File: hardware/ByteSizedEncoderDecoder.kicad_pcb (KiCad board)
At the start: 2 copper layers, 21.6 x 25.4 mm, 17 parts, among them J1 BM04B-SRSS-TB_LF__SN_, J10 1x4 female header pins 0.1", J11 ICSP pads, J2 BM04B-SRSS-TB_LF__SN_, J3 1x4 female header pins 0.1", J4 1x4 female header pins 0.1", J5 1x4 female header pins 0.1", J6 1x4 female header pins 0.1", J7 1x4 female header pins 0.1", J8 1x4 female header pins 0.1", J9 1x4 female header pins 0.1", U1 ATMEGA328PB

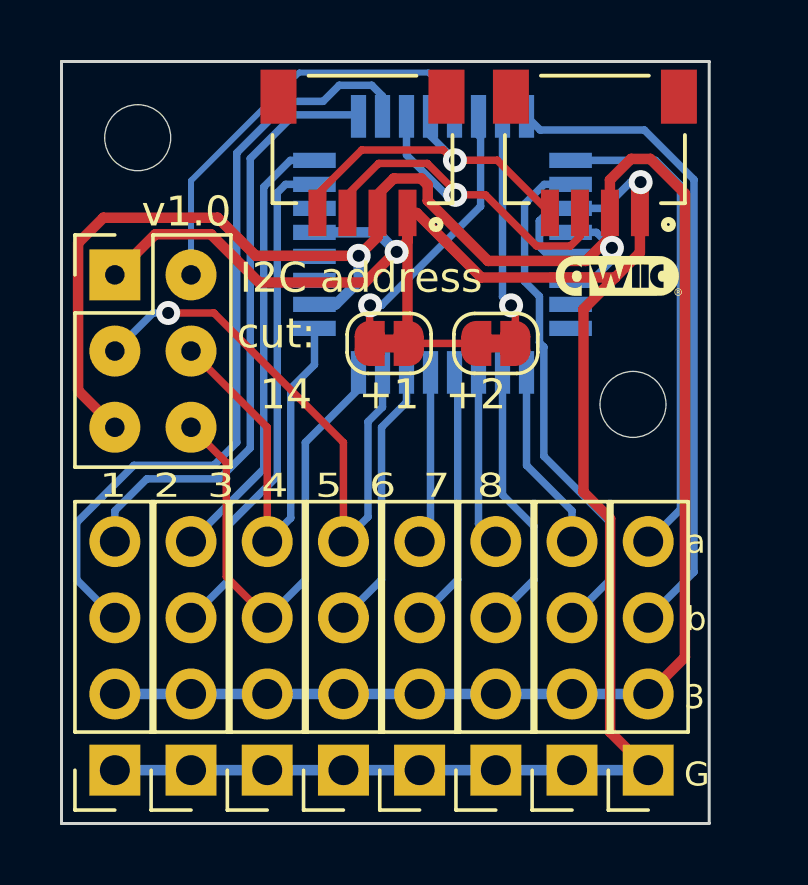
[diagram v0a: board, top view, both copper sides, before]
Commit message: v1.0
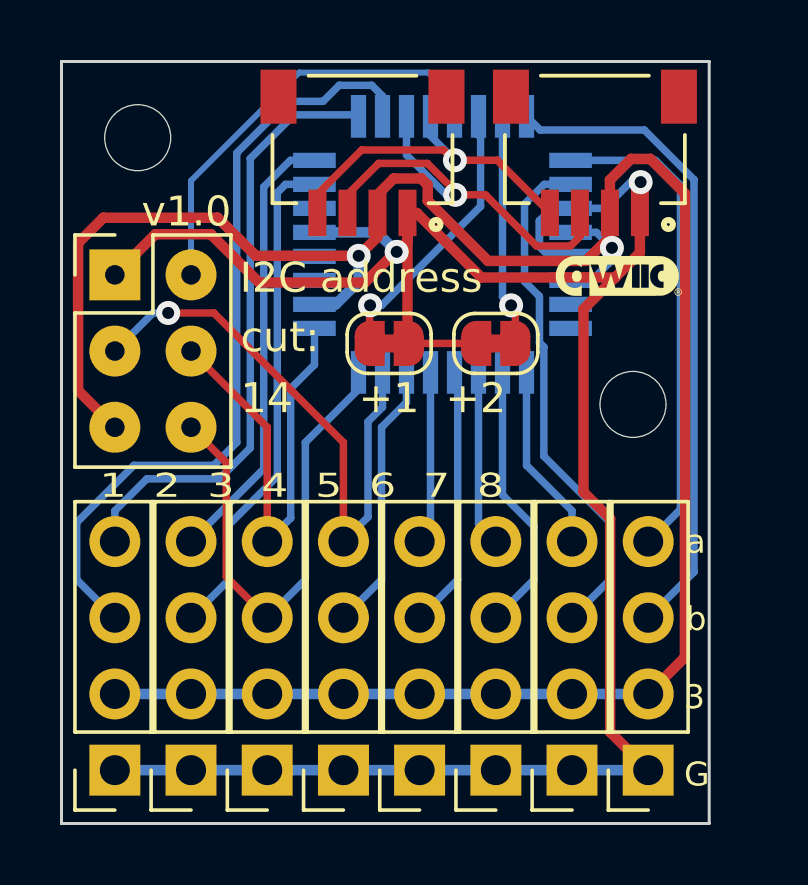
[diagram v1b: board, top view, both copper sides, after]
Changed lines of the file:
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@@
       (plotinvisibletext false)
       (sketchpadsonfab false)
-      (subtractmaskfromsilk false)
+      (subtractmaskfromsilk true)
       (outputformat 1)
       (mirror false)
       (drillshape 0)
       (scaleselection 1)
-      (outputdirectory "C:/Users/Joshua/Desktop/RCM-Hardware-BYTE/gerbers-RCM-Hardware-BYTE-v2.2/")
+      (outputdirectory "gerbers/gerbers - BSCD - v1.0/")
     )
   )
@@
     (effects (font (size 1 1) (thickness 0.15)) (justify left bottom))
   )
-  (gr_text "cut: " (at 159.766 71.374) (layer "F.SilkS")
+  (gr_text "cut: " (at 159.893 71.501) (layer "F.SilkS")
     (effects (font (size 1 1) (thickness 0.15)) (justify left bottom))
   )
@@
     (effects (font (size 1 1) (thickness 0.15)) (justify left bottom))
   )
-  (gr_text "+1  +2" (at 163.83 73.406) (layer "F.SilkS")
+  (gr_text "+1  +2" (at 163.83 73.533) (layer "F.SilkS")
     (effects (font (size 1 1) (thickness 0.15)) (justify left bottom))
   )
@@
     (effects (font (size 0.8 0.8) (thickness 0.15)) (justify left bottom))
   )
-  (gr_text "14\n" (at 160.528 73.406) (layer "F.SilkS")
+  (gr_text "14\n" (at 159.893 73.533) (layer "F.SilkS")
     (effects (font (size 1 1) (thickness 0.15)) (justify left bottom))
   )
